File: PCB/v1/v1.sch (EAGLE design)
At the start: 69 parts, among them U2 AT24C512C-SHD-B

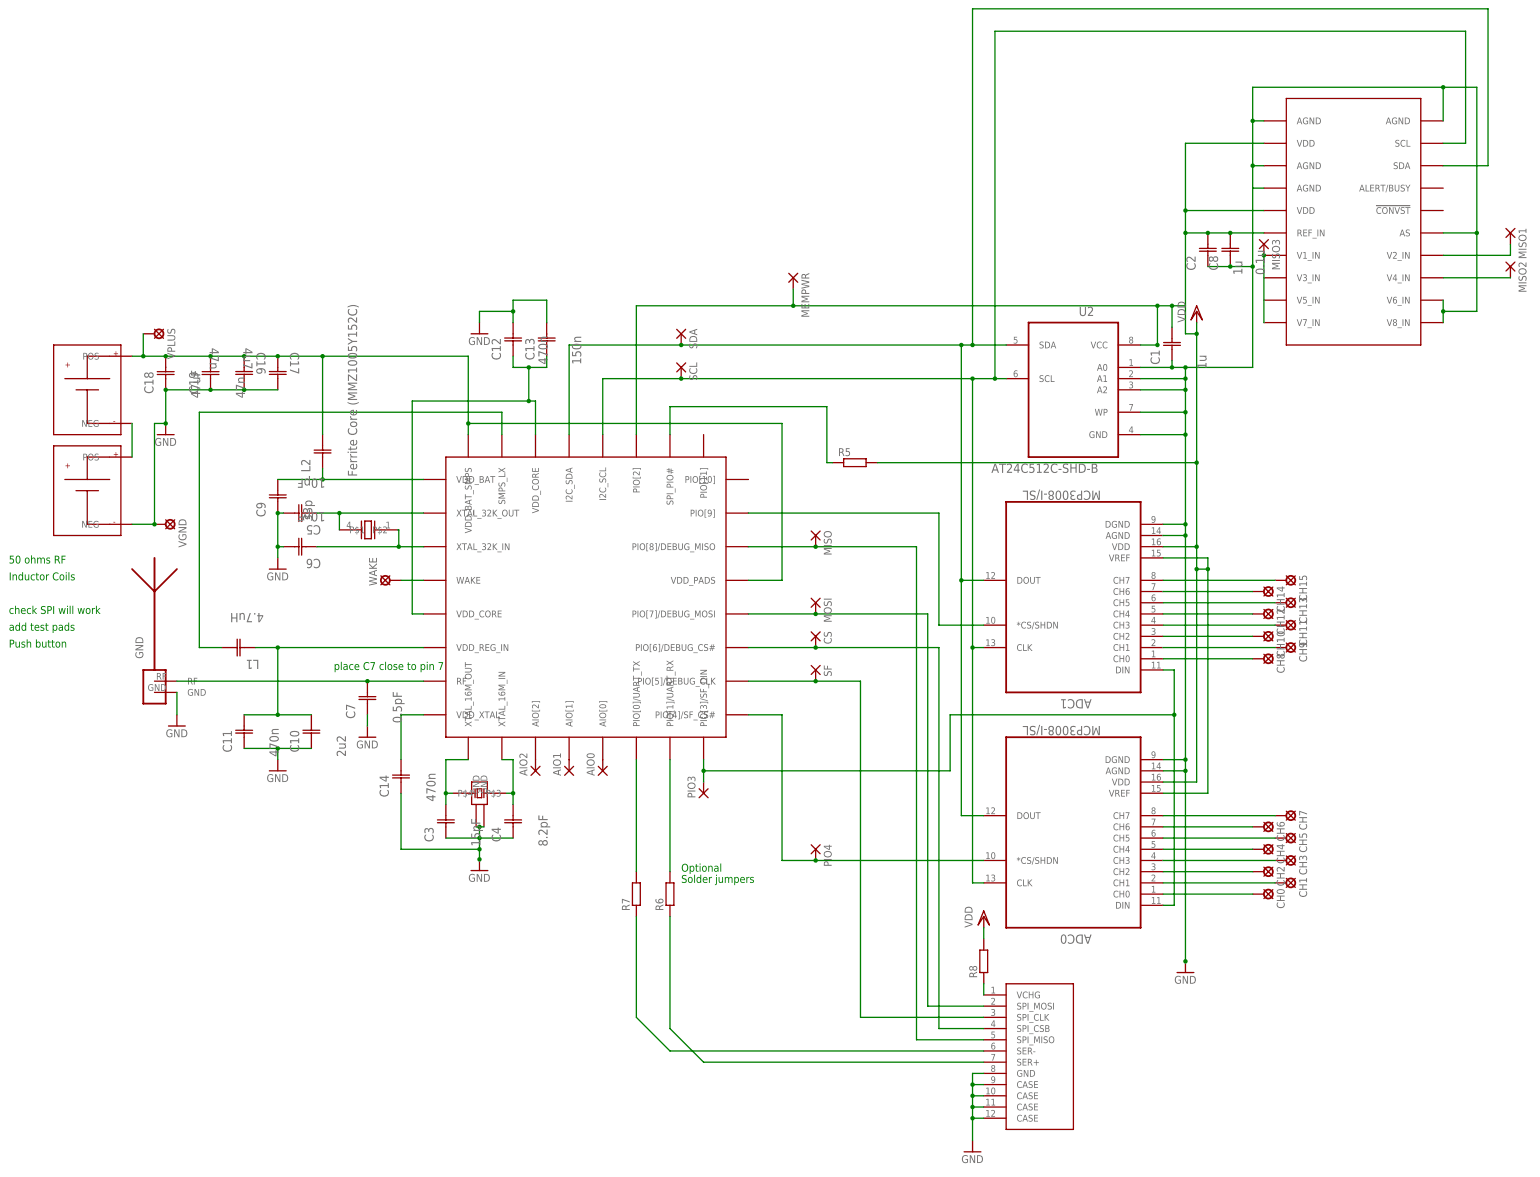
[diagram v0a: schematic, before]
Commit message: do a once over, then fab
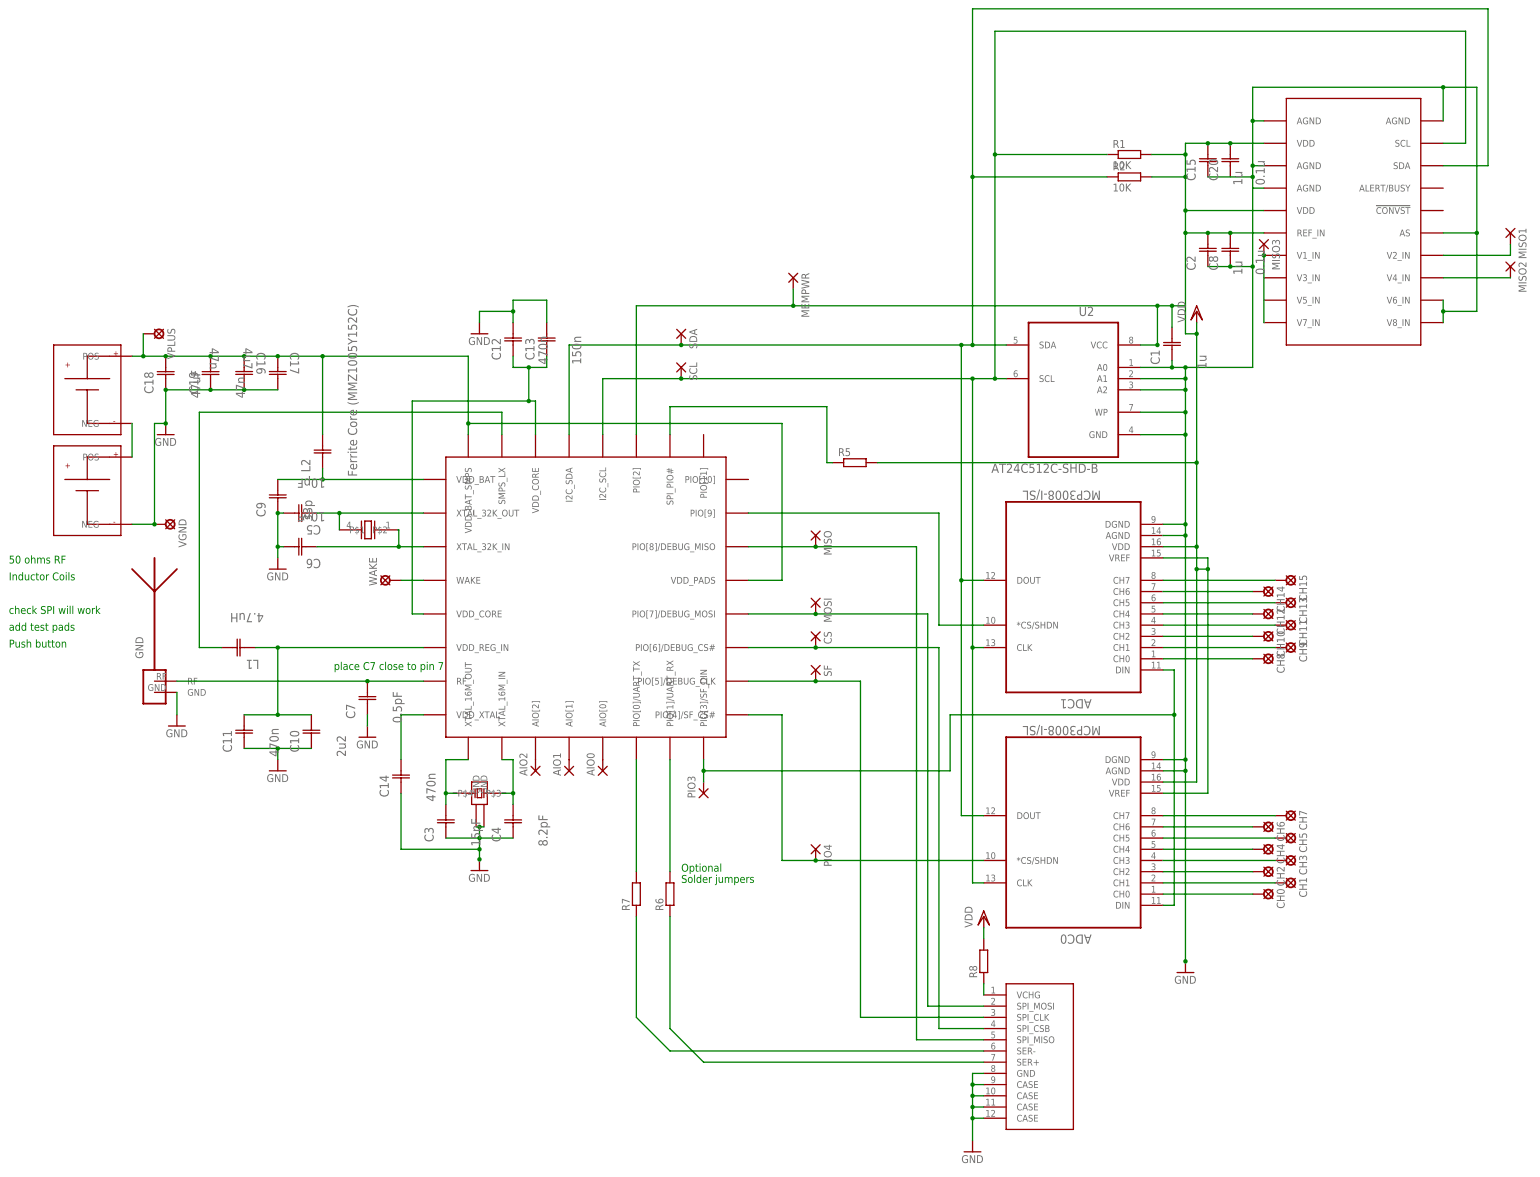
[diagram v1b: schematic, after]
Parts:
- added C15: 1u, AVX_By_element14_Batch_1:UQCL2A100JAT2A/500
- added C20: 0.1u, AVX_By_element14_Batch_1:UQCL2A100JAT2A/500
- added R1, R2: 10K, rcl:R-EU_R0402
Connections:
- net GND: now also C15.C1
- net SCL: now also R1.1
- net SDA: now also R2.1
- net VDD: now also C15.C2, C20.C2, R1.2, R2.2
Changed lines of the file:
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@@
 <part name="MISO2" library="wirepad" deviceset="1,6/0,8" device=""/>
 <part name="MISO3" library="wirepad" deviceset="1,6/0,8" device=""/>
+<part name="R1" library="rcl" deviceset="R-EU_" device="R0402" value="10K"/>
+<part name="R2" library="rcl" deviceset="R-EU_" device="R0402" value="10K"/>
+<part name="C15" library="AVX_By_element14_Batch_1" deviceset="UQCL2A100JAT2A/500" device="" value="1u"/>
+<part name="C20" library="AVX_By_element14_Batch_1" deviceset="UQCL2A100JAT2A/500" device="" value="0.1u"/>
 </parts>
 <sheets>
@@
 <instance part="MISO2" gate="P" x="149.86" y="129.54" rot="R270"/>
 <instance part="MISO3" gate="P" x="93.98" y="134.62" rot="R270"/>
+<instance part="R1" gate="G$1" x="63.5" y="154.94"/>
+<instance part="R2" gate="G$1" x="63.5" y="149.86"/>
+<instance part="C15" gate="A" x="81.28" y="149.86" rot="R90"/>
+<instance part="C20" gate="A" x="86.36" y="149.86" rot="R90"/>
 </instances>
 <busses>
@@
 <wire x1="139.7" y1="157.48" x2="139.7" y2="182.88" width="0.1524" layer="91"/>
 <wire x1="139.7" y1="182.88" x2="33.02" y2="182.88" width="0.1524" layer="91"/>
-<wire x1="33.02" y1="182.88" x2="33.02" y2="104.14" width="0.1524" layer="91"/>
+<wire x1="33.02" y1="182.88" x2="33.02" y2="154.94" width="0.1524" layer="91"/>
 <junction x="33.02" y="104.14"/>
+<pinref part="R1" gate="G$1" pin="1"/>
+<wire x1="33.02" y1="154.94" x2="33.02" y2="104.14" width="0.1524" layer="91"/>
+<wire x1="58.42" y1="154.94" x2="33.02" y2="154.94" width="0.1524" layer="91"/>
+<junction x="33.02" y="154.94"/>
 </segment>
 </net>
@@
 <junction x="25.4" y="111.76"/>
 <pinref part="U$1" gate="G$1" pin="I2C_SDA"/>
-<wire x1="27.94" y1="111.76" x2="27.94" y2="187.96" width="0.1524" layer="91"/>
+<wire x1="27.94" y1="111.76" x2="27.94" y2="149.86" width="0.1524" layer="91"/>
 <junction x="27.94" y="111.76"/>
+<wire x1="27.94" y1="149.86" x2="27.94" y2="187.96" width="0.1524" layer="91"/>
 <wire x1="27.94" y1="187.96" x2="144.78" y2="187.96" width="0.1524" layer="91"/>
 <wire x1="144.78" y1="187.96" x2="144.78" y2="152.4" width="0.1524" layer="91"/>
 <pinref part="U$7" gate="G$1" pin="SDA"/>
 <wire x1="144.78" y1="152.4" x2="134.62" y2="152.4" width="0.1524" layer="91"/>
+<pinref part="R2" gate="G$1" pin="1"/>
+<wire x1="58.42" y1="149.86" x2="27.94" y2="149.86" width="0.1524" layer="91"/>
+<junction x="27.94" y="149.86"/>
 </segment>
 </net>
@@
 <wire x1="93.98" y1="162.56" x2="91.44" y2="162.56" width="0.1524" layer="91"/>
 <wire x1="91.44" y1="162.56" x2="91.44" y2="152.4" width="0.1524" layer="91"/>
-<wire x1="91.44" y1="152.4" x2="91.44" y2="147.32" width="0.1524" layer="91"/>
+<wire x1="91.44" y1="152.4" x2="91.44" y2="149.86" width="0.1524" layer="91"/>
 <pinref part="U$7" gate="G$1" pin="AGND@2"/>
+<wire x1="91.44" y1="149.86" x2="91.44" y2="147.32" width="0.1524" layer="91"/>
 <wire x1="93.98" y1="152.4" x2="91.44" y2="152.4" width="0.1524" layer="91"/>
 <junction x="91.44" y="152.4"/>
@@
 <wire x1="142.24" y1="137.16" x2="142.24" y2="119.38" width="0.1524" layer="91"/>
 <junction x="142.24" y="137.16"/>
+<pinref part="C15" gate="A" pin="C1"/>
+<wire x1="81.28" y1="149.86" x2="91.44" y2="149.86" width="0.1524" layer="91"/>
+<junction x="91.44" y="149.86"/>
 </segment>
 </net>
@@
 <wire x1="76.2" y1="142.24" x2="93.98" y2="142.24" width="0.1524" layer="91"/>
 <pinref part="U$7" gate="G$1" pin="VDD@1"/>
-<wire x1="93.98" y1="157.48" x2="76.2" y2="157.48" width="0.1524" layer="91"/>
-<wire x1="76.2" y1="157.48" x2="76.2" y2="142.24" width="0.1524" layer="91"/>
+<wire x1="93.98" y1="157.48" x2="86.36" y2="157.48" width="0.1524" layer="91"/>
+<wire x1="86.36" y1="157.48" x2="81.28" y2="157.48" width="0.1524" layer="91"/>
+<wire x1="81.28" y1="157.48" x2="76.2" y2="157.48" width="0.1524" layer="91"/>
+<wire x1="76.2" y1="157.48" x2="76.2" y2="154.94" width="0.1524" layer="91"/>
 <junction x="76.2" y="142.24"/>
+<wire x1="76.2" y1="154.94" x2="76.2" y2="149.86" width="0.1524" layer="91"/>
+<wire x1="76.2" y1="149.86" x2="76.2" y2="142.24" width="0.1524" layer="91"/>
 <wire x1="76.2" y1="120.65" x2="76.2" y2="114.3" width="0.1524" layer="91"/>
 <wire x1="76.2" y1="114.3" x2="78.74" y2="114.3" width="0.1524" layer="91"/>
@@
 <pinref part="C8" gate="A" pin="C2"/>
 <junction x="86.36" y="137.16"/>
+<pinref part="C15" gate="A" pin="C2"/>
+<junction x="81.28" y="157.48"/>
+<pinref part="C20" gate="A" pin="C2"/>
+<junction x="86.36" y="157.48"/>
+<pinref part="R1" gate="G$1" pin="2"/>
+<wire x1="68.58" y1="154.94" x2="76.2" y2="154.94" width="0.1524" layer="91"/>
+<junction x="76.2" y="154.94"/>
+<pinref part="R2" gate="G$1" pin="2"/>
+<wire x1="68.58" y1="149.86" x2="76.2" y2="149.86" width="0.1524" layer="91"/>
+<junction x="76.2" y="149.86"/>
 </segment>
 <segment>
@@
 <pinref part="C3" gate="A" pin="C2"/>
 <wire x1="-91.44" y1="17.78" x2="-91.44" y2="10.16" width="0.1524" layer="91"/>
+<pinref part="U$1" gate="G$1" pin="XTAL_16M_OUT"/>
 <wire x1="-91.44" y1="10.16" x2="-91.44" y2="7.62" width="0.1524" layer="91"/>
-<wire x1="-89.916" y1="10.16" x2="-91.44" y2="10.16" width="0.1524" layer="91"/>
+<wire x1="-88.9" y1="10.16" x2="-91.44" y2="10.16" width="0.1524" layer="91"/>
 <junction x="-91.44" y="10.16"/>
-<pinref part="U$1" gate="G$1" pin="XTAL_16M_OUT"/>
 </segment>
 </net>
@@
 <pinref part="C4" gate="A" pin="C2"/>
 <wire x1="-76.2" y1="17.78" x2="-76.2" y2="10.16" width="0.1524" layer="91"/>
+<pinref part="U$1" gate="G$1" pin="XTAL_16M_IN"/>
 <wire x1="-76.2" y1="10.16" x2="-76.2" y2="7.62" width="0.1524" layer="91"/>
-<wire x1="-77.724" y1="10.16" x2="-76.2" y2="10.16" width="0.1524" layer="91"/>
+<wire x1="-78.74" y1="10.16" x2="-76.2" y2="10.16" width="0.1524" layer="91"/>
 <junction x="-76.2" y="10.16"/>
-<pinref part="U$1" gate="G$1" pin="XTAL_16M_IN"/>
-</segment>
-</net>
+</segment>
+</net>
